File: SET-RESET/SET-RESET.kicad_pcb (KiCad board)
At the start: 2 copper layers, 100.1 x 100.1 mm, 113 parts, among them J1 BMS, J2 BSPD, J3 IMD, J4 IMD_SHTDNW, J5 BMS_SHTDNW, J6 BSPD_SHTDNW, J7 Led's paineis, J8 voltage supply, K1 RELAY_19.1x15.5mm, K2 RELAY_19.1x15.5mm, K3 RELAY_19.1x15.5mm, K4 RELAY_19.1x15.5mm, K5 RELAY_19.1x15.5mm, K6 RELAY_19.1x15.5mm, Q1 BC557, Q10 BC548, Q11 BC548, Q12 BC557, Q13 BC548, Q14 BC548, Q15 BC557, Q16 BC548, Q17 BC548, Q18 BC557, Q2 BC557, Q3 BC557, Q4 Si2302DS, Q5 Si2302DS, Q6 Si2302DS, Q7 BC548, Q8 BC548, Q9 BC548, U1 TLP290-4

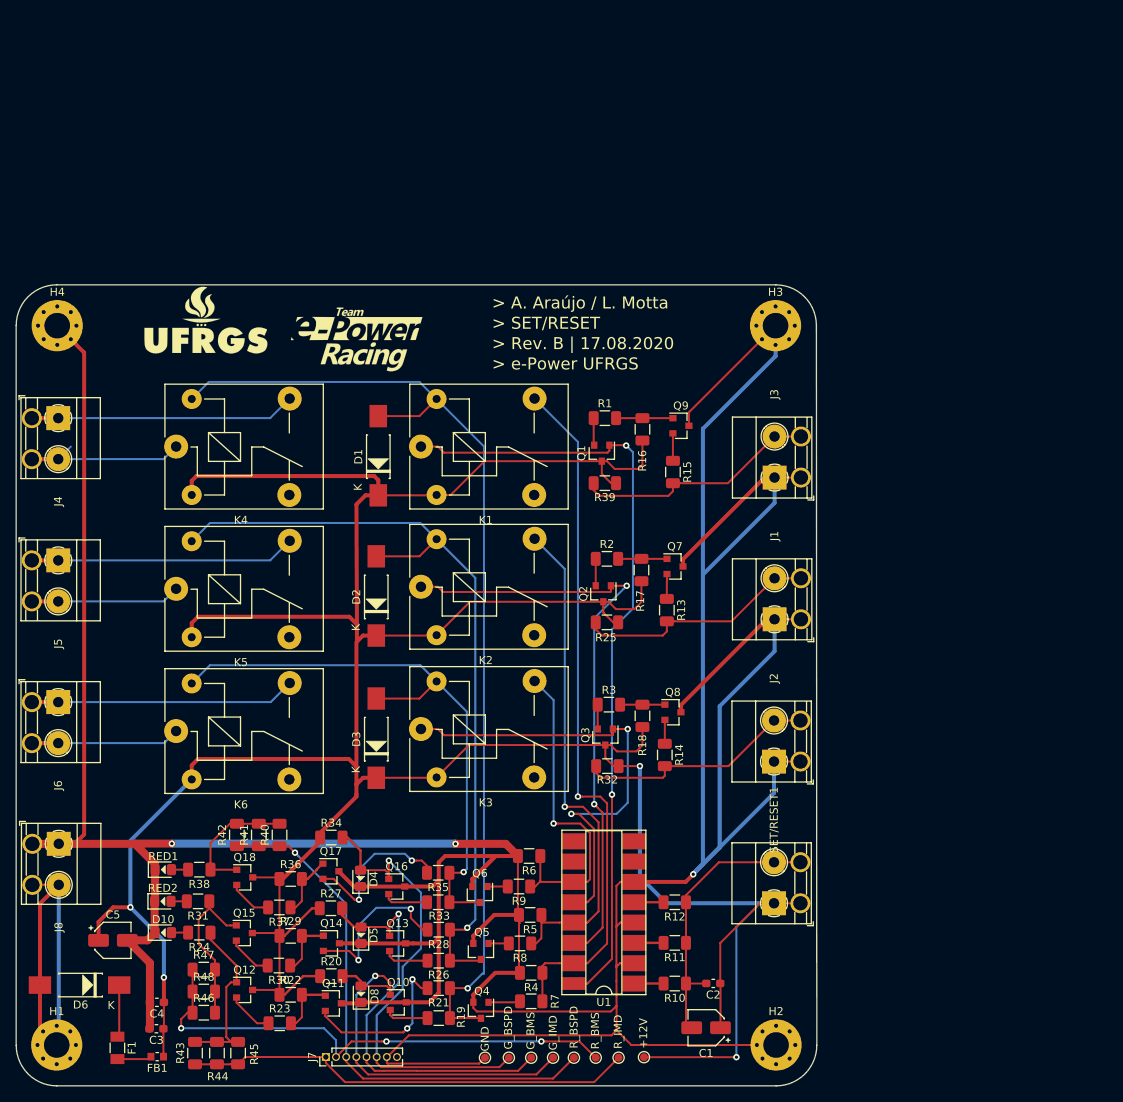
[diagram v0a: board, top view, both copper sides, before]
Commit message: Set/Reset Rev. C
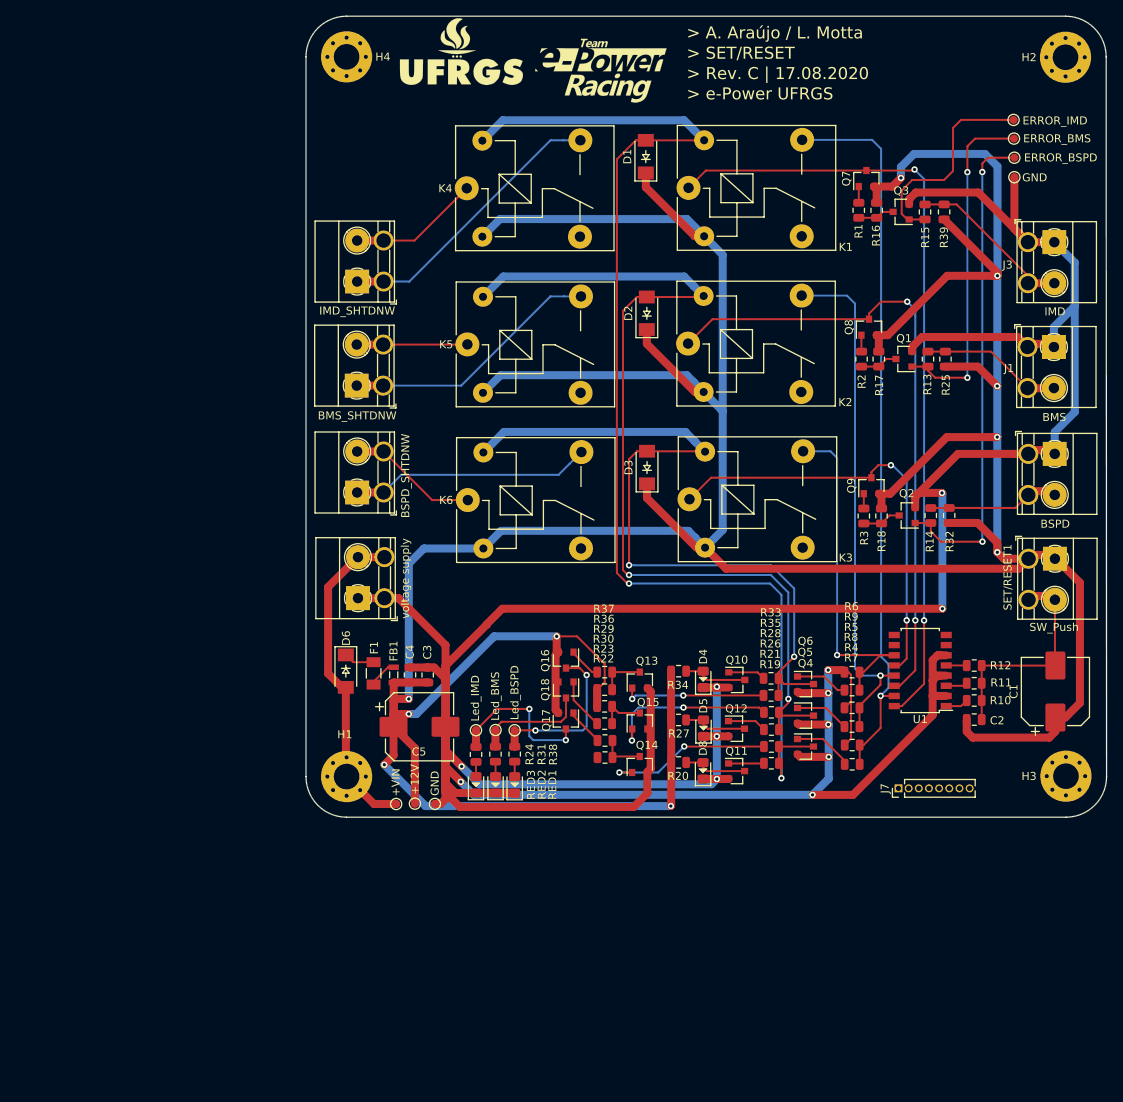
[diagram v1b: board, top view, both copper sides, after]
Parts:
- removed D10: RED, e-Power:LED_0805_1.15x1.40mm_HandSolder
- removed G_BMS1: G_BMS, e-Power:TestPoint_Pad_D1.0mm
- removed G_BSPD1: G_BSPD, e-Power:TestPoint_Pad_D1.0mm
- removed G_IMD1: G_IMD, e-Power:TestPoint_Pad_D1.0mm
- removed R40, R41, R42, R43, R44, R45, R46, R47, R48: 1K, Resistor_SMD:R_1206_3216Metric
- removed R_BMS1: R_BMS, e-Power:TestPoint_Pad_D1.0mm
- removed R_BSPD1: R_BSPD, e-Power:TestPoint_Pad_D1.0mm
- removed R_IMD1: R_IMD, e-Power:TestPoint_Pad_D1.0mm
- added RED3: RED, e-Power:LED_0805_1.15x1.40mm_HandSolder, F.Cu at (170.5, 121.0)
- added TP10: +VIN, e-Power:TestPoint_Pad_D1.0mm, F.Cu at (160.5, 123.4)
- added TP11: GND, e-Power:TestPoint_Pad_D1.0mm, F.Cu at (165.3, 123.4)
- added TP3: ERROR_BMS, e-Power:TestPoint_Pad_D1.0mm, F.Cu at (237.7, 40.2)
- added TP4: ERROR_IMD, e-Power:TestPoint_Pad_D1.0mm, F.Cu at (237.7, 37.9)
- added TP5: ERROR_BSPD, e-Power:TestPoint_Pad_D1.0mm, F.Cu at (237.8, 42.6)
- added TP7: Led_BSPD, e-Power:TestPoint_Pad_D1.0mm, F.Cu at (175.3, 114.2)
- added TP8: Led_IMD, e-Power:TestPoint_Pad_D1.0mm, F.Cu at (170.5, 114.2)
- added TP9: Led_BMS, e-Power:TestPoint_Pad_D1.0mm, F.Cu at (172.9, 114.2)
- C1, C5: footprint Capacitor_SMD:CP_Elec_4x5.3 -> Capacitor_SMD:CP_Elec_8x10
- C2, C3, C4: footprint Capacitor_SMD:C_0603_1608Metric_Pad1.05x0.95mm_HandSolder -> Capacitor_SMD:C_0805_2012Metric
- D1, D2, D3, D6: value 1N5819 -> SS54HF; footprint e-Power:DO-41_SMD -> e-Power:DO-214AC
- FB1: footprint e-Power:FB_0603_1608Metric -> e-Power:FB_0805_2012Metric
- Q1, Q12, Q15, Q18, Q2, Q3: value BC557 -> MMBT5551
- Q10, Q11, Q13, Q14, Q16, Q17, Q7, Q8, Q9: value BC548 -> MMBT5551
- R1, R10, R11, R12, R13, R14, R15, R16, R17, R18, R19, R2, R20, R21, R22, R23, R24, R25, R26, R27, R28, R29, R3, R30, R31, R32, R33, R34, R35, R36, R37, R38, R39, R4, R5, R6, R7, R8, R9: footprint Resistor_SMD:R_1206_3216Metric -> Resistor_SMD:R_0805_2012Metric
- U1: footprint e-Power:TLP290-4 -> e-Power:SOIC-16_4.55x10.3mm_P1.27mm(TLP290-4)
- moved H2 128.7 mm to (244.1, 30.1)
- moved TP1 128.4 mm to (237.8, 45.1), turned to 270 degrees
- moved J7 79.1 mm to (223.3, 121.5)
- moved Q3 75.3 mm to (223.6, 49.4), turned to 180 degrees
- moved Q12 69.6 mm to (203.0, 114.0)
- moved H3 67.0 mm to (244.2, 119.9)
- moved C1 60.6 mm to (242.9, 109.4), turned to 90 degrees
- moved Q10 58.4 mm to (203.1, 107.9)
- moved Q11 58.2 mm to (203.0, 119.3)
- moved F1 56.7 mm to (157.7, 107.1)
- moved FB1 56.1 mm to (160.2, 107.3), turned to 90 degrees
- moved Q15 56.1 mm to (190.9, 113.0), turned to 90 degrees
- moved C3 55.7 mm to (164.4, 107.3), turned to 90 degrees
- moved SET/RESET1 55.6 mm to (242.8, 92.8), turned to 270 degrees
- moved R39 54.3 mm to (229.0, 49.4), turned to 270 degrees
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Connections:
- D4 pad 2: /ledGREEN_BSPD -> Net-(D4-Pad2)
- D5 pad 2: /ledGREEN_BMS -> Net-(D5-Pad2)
- D8 pad 2: /ledGREEN_IMD -> Net-(D8-Pad2)
- J7 pad 1: /ledRED_IMD -> /led_IMD
- J7 pad 2: /ledRED_BMS -> /led_BMS
- J7 pad 3: /ledRED_BSPD -> /led_BSPD
- J7 pad 4: /ledGREEN_IMD -> Net-(J7-Pad4)
- J7 pad 5: /ledGREEN_BMS -> Net-(J7-Pad5)
- J7 pad 6: /ledGREEN_BSPD -> Net-(J7-Pad6)
- Q1 pad 1: Net-(K1-Pad1) -> Net-(Q1-Pad1)
- Q1 pad 2: Net-(Q1-Pad2) -> GND
- Q1 pad 3: +12V -> Net-(Q1-Pad3)
- Q10 pad 1: /ledGREEN_IMD -> Net-(Q10-Pad1)
- Q10 pad 2: Net-(Q10-Pad2) -> GND
- Q10 pad 3: GND -> Net-(D4-Pad2)
- Q11 pad 2: Net-(Q11-Pad2) -> GND
- Q11 pad 3: GND -> Net-(D8-Pad2)
- Q12 pad 2: Net-(Q12-Pad2) -> GND
- Q12 pad 3: +12V -> Net-(D5-Pad2)
- Q13 pad 1: /ledGREEN_BMS -> Net-(Q13-Pad1)
- Q13 pad 2: Net-(Q13-Pad2) -> GND
- Q13 pad 3: GND -> Net-(Q13-Pad3)
- Q14 pad 2: Net-(Q14-Pad2) -> GND
- Q14 pad 3: GND -> Net-(Q14-Pad3)
- Q15 pad 2: Net-(Q15-Pad2) -> GND
- Q15 pad 3: +12V -> Net-(Q15-Pad3)
- Q16 pad 1: /ledGREEN_BSPD -> Net-(Q16-Pad1)
- Q16 pad 2: Net-(Q16-Pad2) -> +12V
- Q16 pad 3: GND -> /led_BSPD
- Q17 pad 2: Net-(Q17-Pad2) -> +12V
- Q17 pad 3: GND -> /led_IMD
- Q18 pad 2: Net-(Q18-Pad2) -> +12V
- Q18 pad 3: +12V -> /led_BMS
- Q2 pad 1: Net-(K2-Pad1) -> Net-(Q2-Pad1)
- Q2 pad 2: Net-(Q2-Pad2) -> GND
- Q2 pad 3: +12V -> Net-(Q2-Pad3)
- Q3 pad 1: Net-(K3-Pad1) -> Net-(Q3-Pad1)
- Q3 pad 2: Net-(Q3-Pad2) -> GND
- Q3 pad 3: +12V -> Net-(Q3-Pad3)
- Q7 pad 2: Net-(Q7-Pad2) -> +12V
- Q7 pad 3: GND -> Net-(K1-Pad1)
- Q8 pad 2: Net-(Q8-Pad2) -> +12V
- Q8 pad 3: GND -> Net-(K2-Pad1)
- Q9 pad 2: Net-(Q9-Pad2) -> +12V
- Q9 pad 3: GND -> Net-(K3-Pad1)
- R1 pad 1: Net-(Q1-Pad2) -> Net-(Q7-Pad1)
- R1 pad 2: Net-(Q9-Pad1) -> Net-(Q3-Pad3)
- R13 pad 1: Net-(Q7-Pad2) -> Net-(Q1-Pad1)
- R14 pad 1: Net-(Q8-Pad2) -> Net-(Q2-Pad1)
- R15 pad 1: Net-(Q9-Pad2) -> Net-(Q3-Pad1)
- R16 pad 2: Net-(Q9-Pad1) -> Net-(Q3-Pad3)
- R17 pad 2: Net-(Q7-Pad1) -> Net-(Q1-Pad3)
- R18 pad 2: Net-(Q8-Pad1) -> Net-(Q2-Pad3)
- R19 pad 1: Net-(Q10-Pad2) -> Net-(Q11-Pad1)
- R2 pad 1: Net-(Q2-Pad2) -> Net-(Q8-Pad1)
- R2 pad 2: Net-(Q7-Pad1) -> Net-(Q1-Pad3)
- R20 pad 2: /ledGREEN_IMD -> Net-(D8-Pad2)
- R21 pad 2: Net-(Q11-Pad2) -> Net-(Q14-Pad1)
- R22 pad 2: Net-(Q11-Pad1) -> Net-(Q14-Pad3)
- R23 pad 1: Net-(Q12-Pad2) -> Net-(Q17-Pad1)
- R23 pad 2: Net-(Q11-Pad1) -> Net-(Q14-Pad3)
- R24 pad 1: Net-(Q12-Pad1) -> /led_IMD
- R26 pad 1: Net-(Q13-Pad2) -> Net-(Q12-Pad1)
- R27 pad 2: /ledGREEN_BMS -> Net-(D5-Pad2)
- R28 pad 1: Net-(Q14-Pad2) -> Net-(Q15-Pad1)
- R29 pad 2: Net-(Q14-Pad1) -> Net-(Q15-Pad3)
- R3 pad 1: Net-(Q3-Pad2) -> Net-(Q9-Pad1)
- R3 pad 2: Net-(Q8-Pad1) -> Net-(Q2-Pad3)
- R30 pad 1: Net-(Q14-Pad1) -> Net-(Q15-Pad3)
- R30 pad 2: Net-(Q15-Pad2) -> Net-(Q18-Pad1)
- R31 pad 1: Net-(Q15-Pad1) -> /led_BMS
- R33 pad 1: Net-(Q16-Pad2) -> Net-(Q10-Pad1)
- R34 pad 2: /ledGREEN_BSPD -> Net-(D4-Pad2)
- R35 pad 2: Net-(Q17-Pad2) -> Net-(Q13-Pad1)
- R36 pad 2: Net-(Q17-Pad1) -> Net-(Q13-Pad3)
- R37 pad 1: Net-(Q17-Pad1) -> Net-(Q13-Pad3)
- R37 pad 2: Net-(Q18-Pad2) -> Net-(Q16-Pad1)
- R38 pad 1: Net-(Q18-Pad1) -> /led_BSPD
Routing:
- net +12V: track 435.3 -> 551.5 mm, vias 4 -> 10
- net GND: track 587.9 -> 494.2 mm, vias 3 -> 12
- net /ledRED_BSPD: track 66.8 -> 0.00 mm, vias 1 -> 0
- net /ledRED_BMS: track 64.5 -> 0.00 mm, vias 3 -> 0
- net Net-(Q2-Pad1): track 0.00 -> 61.6 mm, vias 0 -> 2
- net /ledGREEN_BSPD: track 58.5 -> 0.00 mm, vias 1 -> 0
- net /ledRED_IMD: track 56.3 -> 0.00 mm
- net /ledGREEN_BMS: track 52.8 -> 0.00 mm, vias 1 -> 0
- net /ledGREEN_IMD: track 48.6 -> 0.00 mm, vias 1 -> 0
- net Net-(Q1-Pad1): track 0.00 -> 43.0 mm, vias 0 -> 2
- net Net-(Q3-Pad1): track 0.00 -> 26.9 mm
- net Net-(Q11-Pad2): track 20.9 -> 0.00 mm, vias 2 -> 0
- net /led_BSPD: track 0.00 -> 20.7 mm, vias 0 -> 2
- net Net-(Q14-Pad2): track 20.5 -> 0.00 mm, vias 2 -> 0
- net Net-(Q17-Pad2): track 20.2 -> 0.00 mm, vias 2 -> 0
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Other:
- board text added: "> Rev. C | 17.08.2020"
- board text removed: "> Rev. B | 17.08.2020"
